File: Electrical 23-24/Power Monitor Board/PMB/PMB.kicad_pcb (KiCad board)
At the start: 2 copper layers, 16 parts, among them J1 Conn_01x03_Pin

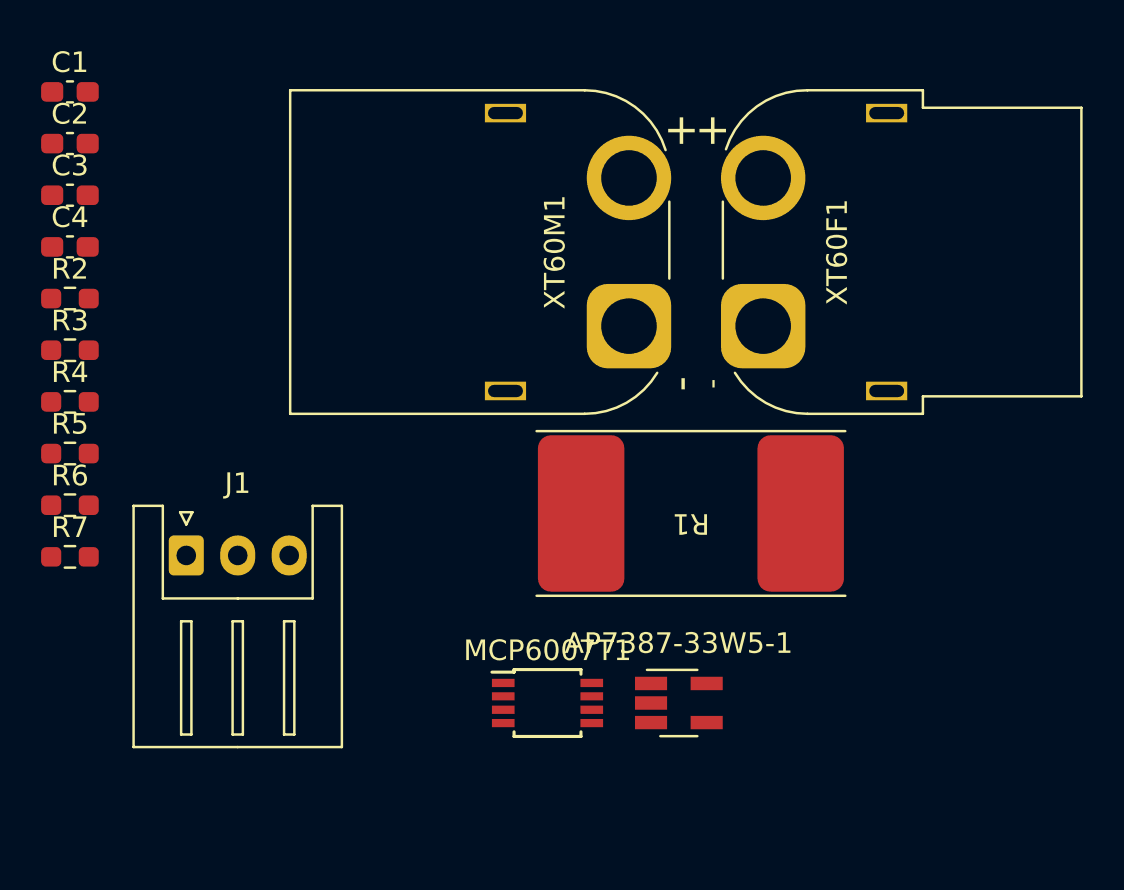
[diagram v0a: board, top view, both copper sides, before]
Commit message: Finish PMB
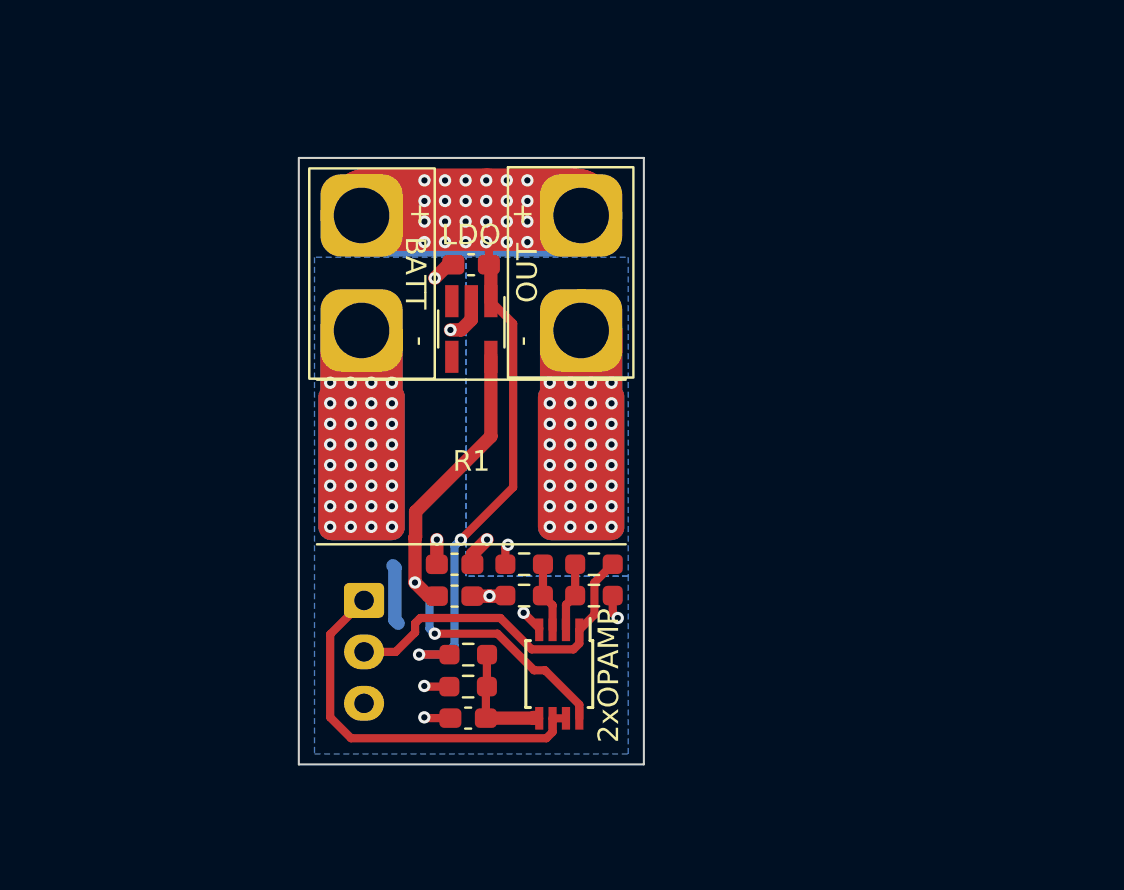
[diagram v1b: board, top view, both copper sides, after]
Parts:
- removed XT60F1: ~, Connector_AMASS:AMASS_XT60PW-F_1x02_P7.20mm_Horizontal
- removed XT60M1: XT60M, Connector_AMASS:AMASS_XT60PW-M_1x02_P7.20mm_Horizontal
- added BATT1: XT60M, PMB:Power, F.Cu at (151.6, 84.8)
- added OUT1: ~, PMB:Power, F.Cu at (162.3, 84.8)
- J1: moved to B.Cu
- moved C1 36.1 mm to (156.8, 106.5), turned to 180 degrees
- moved C2 28.9 mm to (156.2, 100.5), turned to 180 degrees
- moved R2 26.0 mm to (156.8, 103.4)
- moved R6 25.8 mm to (162.9, 100.5), turned to 180 degrees
- moved R7 25.5 mm to (162.9, 99.0)
- moved R3 25.3 mm to (156.8, 104.9), turned to 180 degrees
- moved C4 24.2 mm to (156.2, 99.0), turned to 180 degrees
- moved R4 23.4 mm to (159.5, 99.0)
- moved R5 23.1 mm to (159.5, 100.5), turned to 180 degrees
- moved AP7387-33W5-1 20.8 mm to (157.0, 87.6), turned to -90 degrees
- moved C3 19.8 mm to (157.0, 84.4), turned to 180 degrees
- moved R1 11.0 mm to (157.0, 94.0)
- moved J1 8.91 mm to (151.8, 100.7), turned to -90 degrees
- moved MCP6007T1 1.52 mm to (161.2, 104.3), turned to -90 degrees
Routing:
- net /BATT: track 0.00 -> 47.8 mm, vias 0 -> 26
- net /GND: track 0.00 -> 28.4 mm, vias 0 -> 40
- net /3V3: track 0.00 -> 25.8 mm, vias 0 -> 2
- net /VM: track 0.00 -> 19.0 mm
- net /GND2: track 0.00 -> 16.8 mm, vias 0 -> 34
- net /CM: track 0.00 -> 16.7 mm
- net /VDIV: track 0.00 -> 5.73 mm
- net Net-(MCP6007T1-+-Pad3): track 0.00 -> 3.38 mm
- net Net-(MCP6007T1---Pad2): track 0.00 -> 3.37 mm
- added copper zone on B.Cu, net /GND
- added copper zone on B.Cu, net /GND2
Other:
- board outline added: 16.8 x 29.5 mm
- board text added: "2xOPAMP"
- board text added: "BATT"
- board text added: "LDO"
- board text added: "OUT"

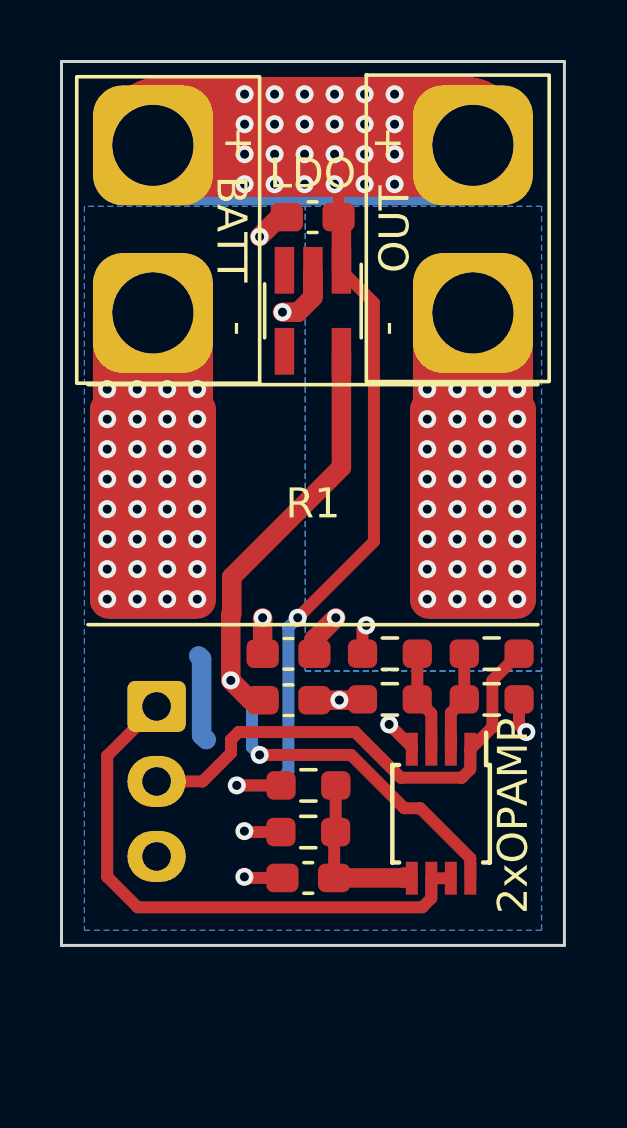
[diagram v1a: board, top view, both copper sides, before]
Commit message: Final PMB
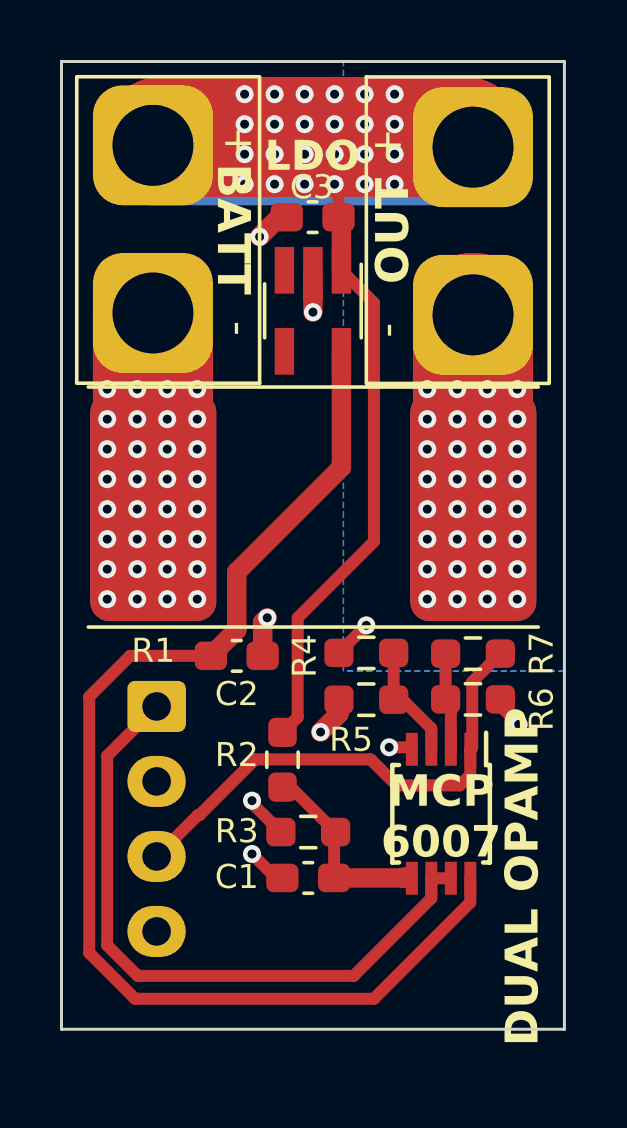
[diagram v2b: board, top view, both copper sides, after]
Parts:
- removed C4: 10uF, Capacitor_SMD:C_0603_1608Metric_Pad1.08x0.95mm_HandSolder
- added G***: LOGO, LOGO, B.Cu at (157.1, 88.7)
- BATT1: value XT60M -> 10AWG_1x02
- J1: value Conn_01x03_Pin -> JST_XH_04; footprint Connector_JST:JST_XH_S3B-XH-A_1x03_P2.50mm_Horizontal -> Connector_JST:JST_XH_S4B-XH-A_1x04_P2.50mm_Horizontal
- OUT1: value ~ -> 10AWG_1x02
- R2: value 150k -> 180k
- R5, R7: value 680k -> 620k
- moved C2 2.27 mm to (154.4, 99.1)
- moved R2 1.22 mm to (156.0, 102.5), turned to -90 degrees
- moved R4 0.79 mm to (158.8, 99.0)
- moved R5 0.78 mm to (158.8, 100.5)
- moved R6 0.62 mm to (162.3, 100.5)
- moved R7 0.62 mm to (162.3, 99.0)
- moved R1 0.08 mm to (157.0, 94.1)
- moved OUT1 0.06 mm to (162.3, 84.9)
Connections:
- J1 pad 2: /CM -> /GND
- J1 pad 3: /GND -> /CM
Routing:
- net /3V3: track 25.8 -> 40.6 mm, vias 2 -> 0
- net /BATT: track 47.8 -> 43.2 mm, vias 26 -> 24
- net /GND: track 28.4 -> 24.3 mm
- net /VM: track 19.0 -> 22.3 mm
- net /GND2: track 16.8 -> 15.9 mm, vias 34 -> 33
- net /VDIV: track 5.73 -> 6.57 mm
- net Net-(MCP6007T1-+-Pad3): track 3.38 -> 3.90 mm
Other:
- board size 16.8 x 29.5 mm -> 16.8 x 32.3 mm
- board text added: "3/15/24"
- board text added: "Ari B Solomiia K"
- board text added: "DUAL OPAMP"
- board text added: "MCP 6007"
- board text added: "VM GND CM GND JST-XH"
- board text removed: "2xOPAMP"
